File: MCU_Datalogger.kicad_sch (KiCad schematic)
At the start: 25 parts

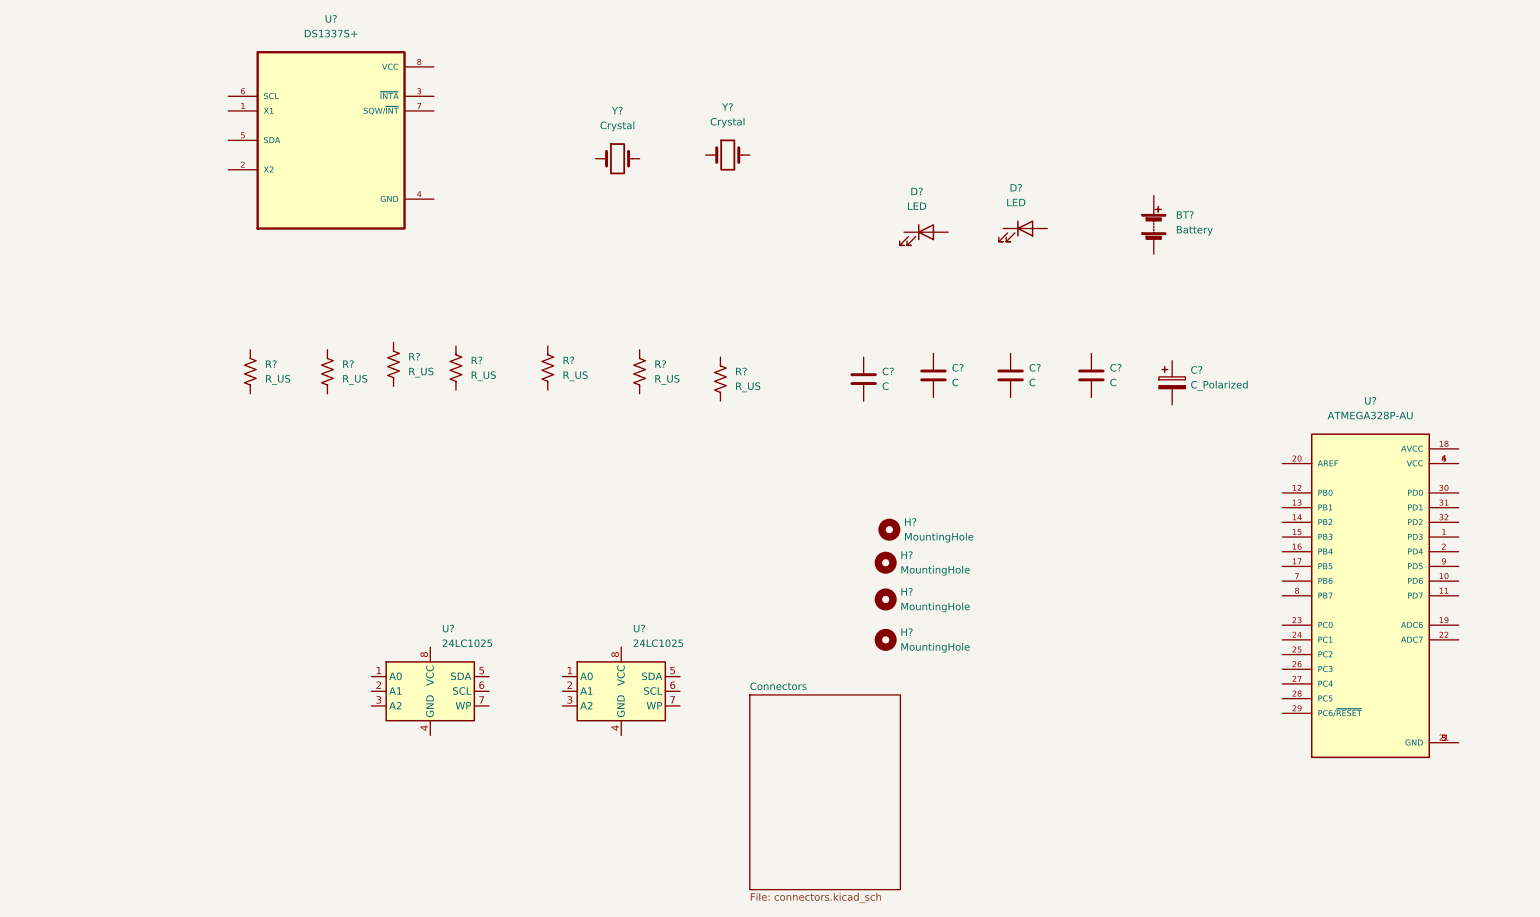
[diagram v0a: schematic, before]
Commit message: Schematic design complete
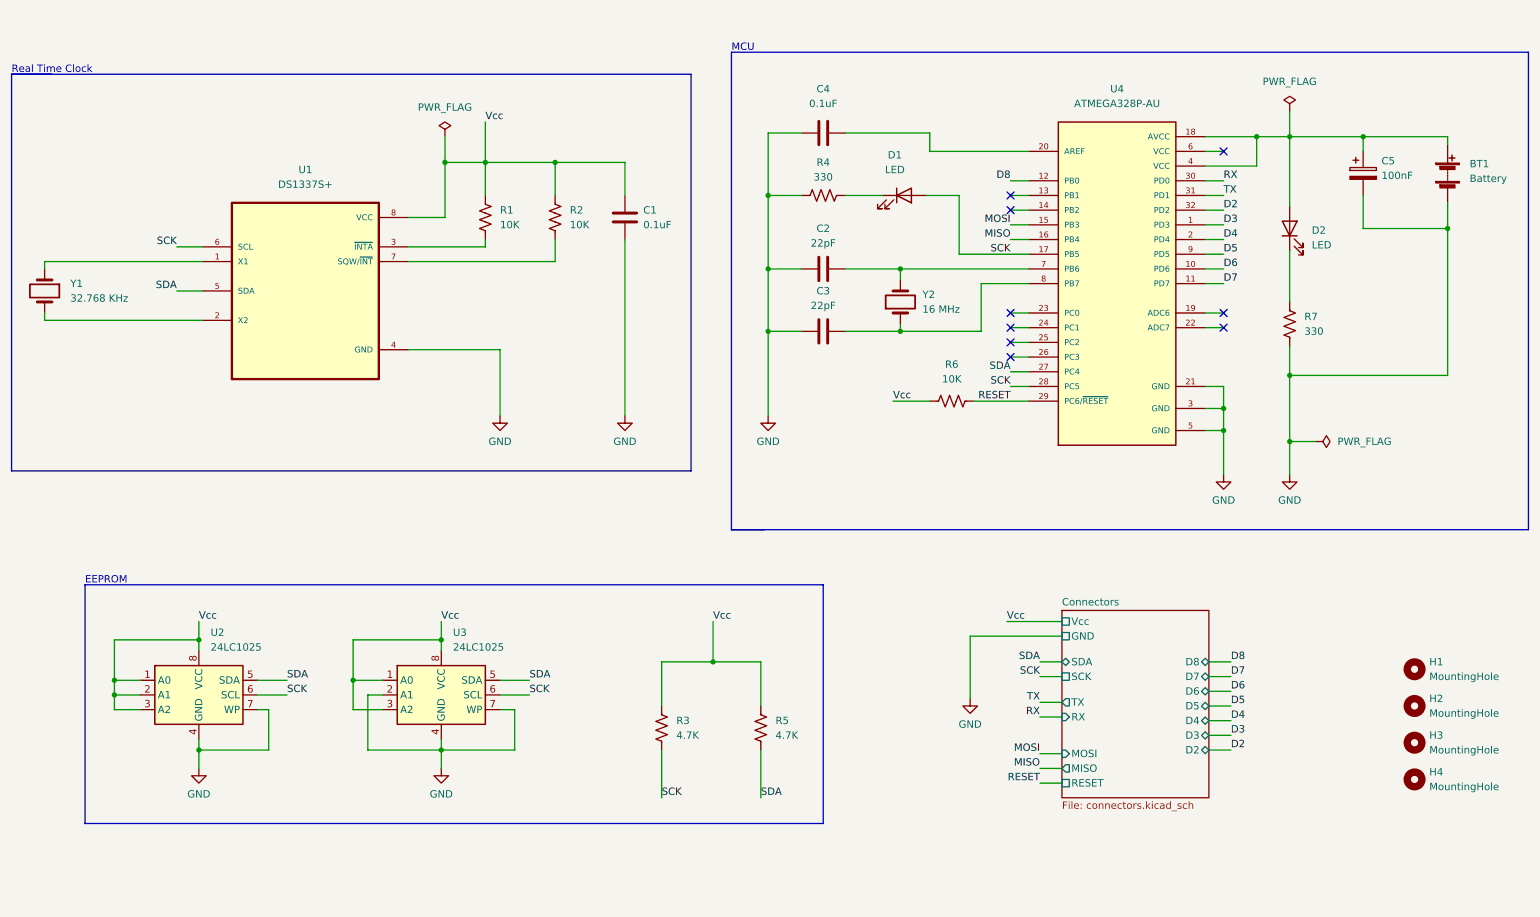
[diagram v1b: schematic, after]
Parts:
- BT1: renamed from BT?; footprint (none) -> Connector_PinHeader_2.54mm:PinHeader_1x02_P2.54mm_Vertical
- C1, C4: renamed from C?; value C -> 0.1uF; footprint (none) -> Capacitor_SMD:C_0805_2012Metric_Pad1.18x1.45mm_HandSolder
- C2, C3: renamed from C?; value C -> 22pF; footprint (none) -> Capacitor_SMD:C_0805_2012Metric_Pad1.18x1.45mm_HandSolder
- C5: renamed from C?; value C_Polarized -> 100nF; footprint (none) -> Capacitor_SMD:C_0805_2012Metric_Pad1.18x1.45mm_HandSolder
- D1, D2: renamed from D?; footprint (none) -> LED_SMD:LED_0805_2012Metric_Pad1.15x1.40mm_HandSolder
- H1, H2, H3, H4: renamed from H?; footprint (none) -> MountingHole:MountingHole_2.1mm
- R1, R2, R6: renamed from R?; value R_US -> 10K; footprint (none) -> Resistor_SMD:R_0805_2012Metric_Pad1.20x1.40mm_HandSolder
- R3, R5: renamed from R?; value R_US -> 4.7K; footprint (none) -> Resistor_SMD:R_0805_2012Metric_Pad1.20x1.40mm_HandSolder
- R4, R7: renamed from R?; value R_US -> 330; footprint (none) -> Resistor_SMD:R_0805_2012Metric_Pad1.20x1.40mm_HandSolder
- U1: renamed from U?; footprint SOIC127P600X175-8N -> DS1337S_:SOIC127P600X175-8N
- U2, U3: renamed from U?; footprint (none) -> Package_SO:SOIC-8_5.23x5.23mm_P1.27mm
- U4: renamed from U?; footprint QFP80P900X900X120-32N -> ATMEGA328P-AU:QFP80P900X900X120-32N
- Y1: renamed from Y?; value Crystal -> 32.768 KHz; footprint (none) -> Crystal:Crystal_SMD_5032-2Pin_5.0x3.2mm_HandSoldering
- Y2: renamed from Y?; value Crystal -> 16 MHz; footprint (none) -> Crystal:Crystal_SMD_5032-2Pin_5.0x3.2mm_HandSoldering
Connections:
- net Vcc: now reaches R5.1
- net Vcc: now also C1.1, R1.1, R2.1, R3.1, R6.1, U1.8 (VCC), U2.1 (A0), U2.2 (A1), U2.3 (A2), U2.8 (VCC), U3.1 (A0), U3.3 (A2), U3.8 (VCC)
- net SDA: now reaches R5.2
- net SDA: now also U1.5 (SDA), U2.5 (SDA), U3.5 (SDA), U4.27 (PC4)
- net GND: now reaches C1.2
- net GND: now also BT1.2 (-), C2.1, C3.1, C4.1, C5.2, R4.1, R7.2, U1.4 (GND), U2.4 (GND), U2.7 (WP), U3.2 (A1), U3.4 (GND), U3.7 (WP), U4.21 (GND), U4.3 (GND), U4.5 (GND)
- net SCK: now reaches U2.6 (SCL)
- net SCK: now also D1.2 (A), R3.2, U1.6 (SCL), U3.6 (SCL), U4.17 (PB5), U4.28 (PC5)
- net at D1.1 (K): now also R4.2
- net at R7.1: now also D2.1 (K)
- net at U1.1 (X1): now also Y1.1
- net at U1.2 (X2): now also Y1.2
- net at U1.3 (~{INTA}): now also R1.2
- net at U1.7 (SQW/~{INT}): now also R2.2
- net at Y2.1: now also C3.2, U4.8 (PB7)
- net at Y2.2: now also C2.2, U4.7 (PB6)
- net D3: now reaches U4.1 (PD3)
- net D6: now reaches U4.10 (PD6)
- net D7: now reaches U4.11 (PD7)
- net D8: now reaches U4.12 (PB0)
- net MOSI: now reaches U4.15 (PB3)
- net MISO: now reaches U4.16 (PB4)
- net at U4.18 (AVCC): now also BT1.1 (+), C5.1, D2.2 (A), U4.4 (VCC)
- net D4: now reaches U4.2 (PD4)
- net at U4.20 (AREF): now also C4.2
- net RESET: now reaches U4.29 (PC6/~{RESET})
- net RESET: now also R6.2
- net RX: now reaches U4.30 (PD0)
- net TX: now reaches U4.31 (PD1)
- net D2: now reaches U4.32 (PD2)
- net at U4.6 (VCC): no longer U4.4 (VCC)
- net D5: now reaches U4.9 (PD5)
- no-connect marks 0 -> 9
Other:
- sheet Connectors ports: added D2, D3, D4, D5, D6, D7, D8, GND, MISO, MOSI, RESET, RX, SCK, SDA, TX, Vcc; removed none
- note added: "EEPROM"
- note added: "MCU"
- note added: "Real Time Clock"
- moved on the sheet: BT1, C1, C2, C3, C4, C5, D1, D2, H1, H2, H3, H4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
